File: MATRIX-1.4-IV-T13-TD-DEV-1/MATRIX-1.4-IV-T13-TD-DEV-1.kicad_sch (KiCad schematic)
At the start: 163 parts, among them Q401 MPSA42, Q402 MPSA42, Q403 MPSA92, Q404 MPSA92, Q405 MJE340, Q406 MJE350, Q407 MJE350, Q408 MJE340, Q409 MJE15032, Q410 MJE15033, Q411 2SC5200, Q412 2SA1943, Q4131 2SC5200, Q41310 2SC5200, Q4132 2SC5200, Q4133 2SC5200, Q4134 2SC5200, Q4135 2SC5200, Q4136 2SC5200, Q4137 2SC5200, Q4138 2SC5200, Q4139 2SC5200, Q4141 2SA1943, Q41410 2SA1943, Q4142 2SA1943, Q4143 2SA1943, Q4144 2SA1943, Q4145 2SA1943, Q4146 2SA1943, Q4147 2SA1943, Q4148 2SA1943, Q4149 2SA1943, Q601 2N5401, Q602 MJE340, Q603 MJE15032, Q604 2SC5200, Q605 2N5401, Q606 MJE340, Q607 2N5401, Q608 2N5401, Q701 2N5551, Q702 MJE350, Q703 MJE15033, Q704 2SA1943, Q705 2N5551, Q706 MJE350, Q707 2N5551, Q708 2N5551

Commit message: Routine Update Fri Jul 15 09:37:09 AM WIB 2022
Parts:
- L601, L701: footprint (none) -> MATRIX_1.4:TOROIDAL_INDUCTOR_0077083A7
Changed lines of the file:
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@@
     (stroke (width 0) (type default) (color 0 0 0 0))
   )
-  (wire (pts (xy 234.95 55.88) (xy 234.95 63.5))
-    (stroke (width 0) (type default) (color 0 0 0 0))
-  )
   (wire (pts (xy 63.5 181.61) (xy 63.5 184.15))
     (stroke (width 0) (type default) (color 0 0 0 0))
@@
     (stroke (width 0) (type default) (color 0 0 0 0))
   )
+  (wire (pts (xy 234.95 55.88) (xy 234.95 63.5))
+    (stroke (width 0) (type default) (color 0 0 0 0))
+  )
   (wire (pts (xy 317.5 111.76) (xy 317.5 115.57))
     (stroke (width 0) (type default) (color 0 0 0 0))
@@
     (property "Reference" "L701" (id 0) (at 336.55 157.48 90))
     (property "Value" "10uH" (id 1) (at 336.55 160.02 90))
-    (property "Footprint" "" (id 2) (at 336.55 152.4 0)
+    (property "Footprint" "MATRIX_1.4:TOROIDAL_INDUCTOR_0077083A7" (id 2) (at 336.55 152.4 0)
       (effects (font (size 1.27 1.27)) hide)
     )
@@
     (property "Reference" "L601" (id 0) (at 336.55 43.18 90))
     (property "Value" "10uH" (id 1) (at 336.55 45.72 90))
-    (property "Footprint" "" (id 2) (at 336.55 50.8 0)
+    (property "Footprint" "MATRIX_1.4:TOROIDAL_INDUCTOR_0077083A7" (id 2) (at 336.55 50.8 0)
       (effects (font (size 1.27 1.27)) hide)
     )

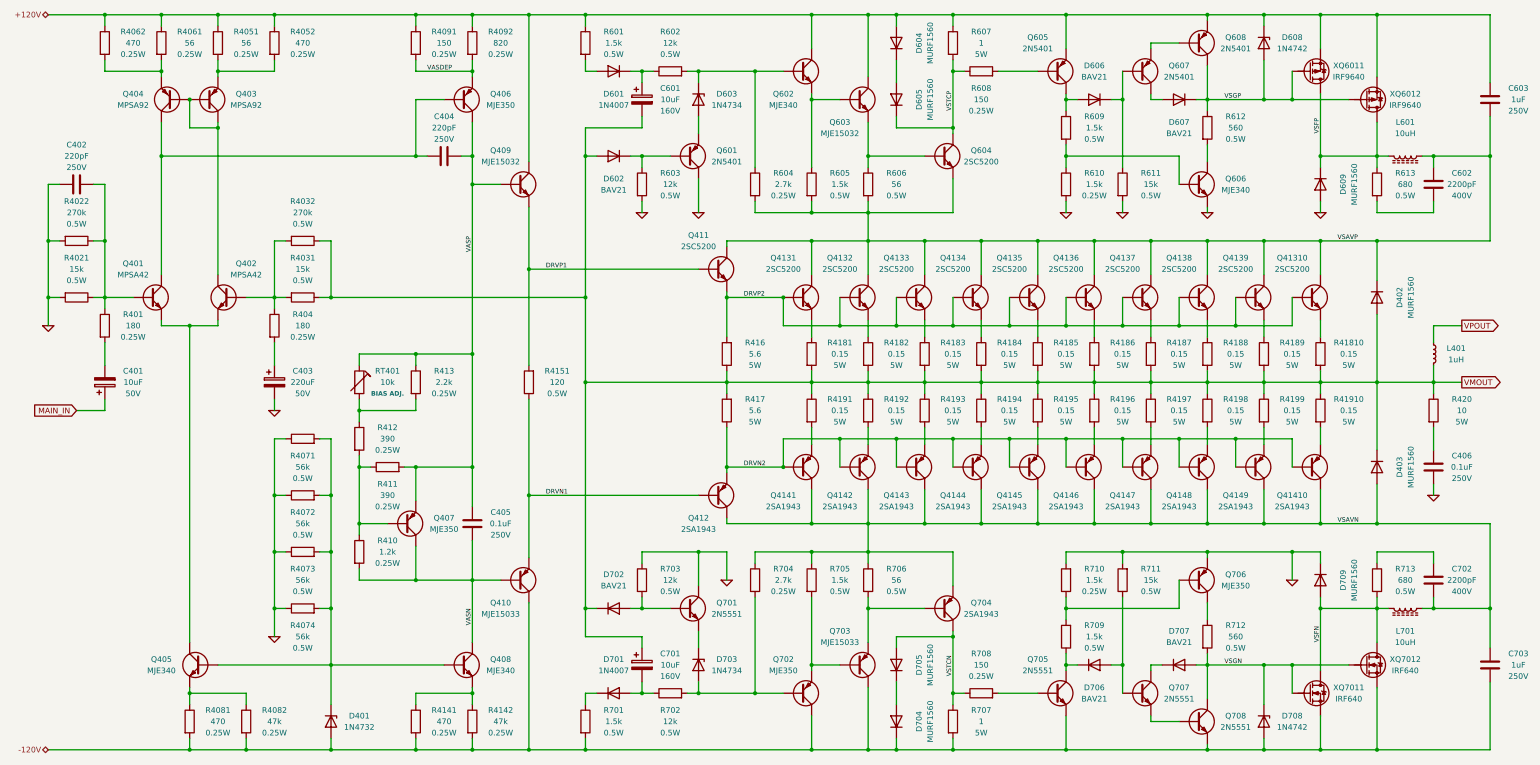
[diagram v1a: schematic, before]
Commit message: Routine Update Sat Jul 16 10:11:34 AM WIB 2022
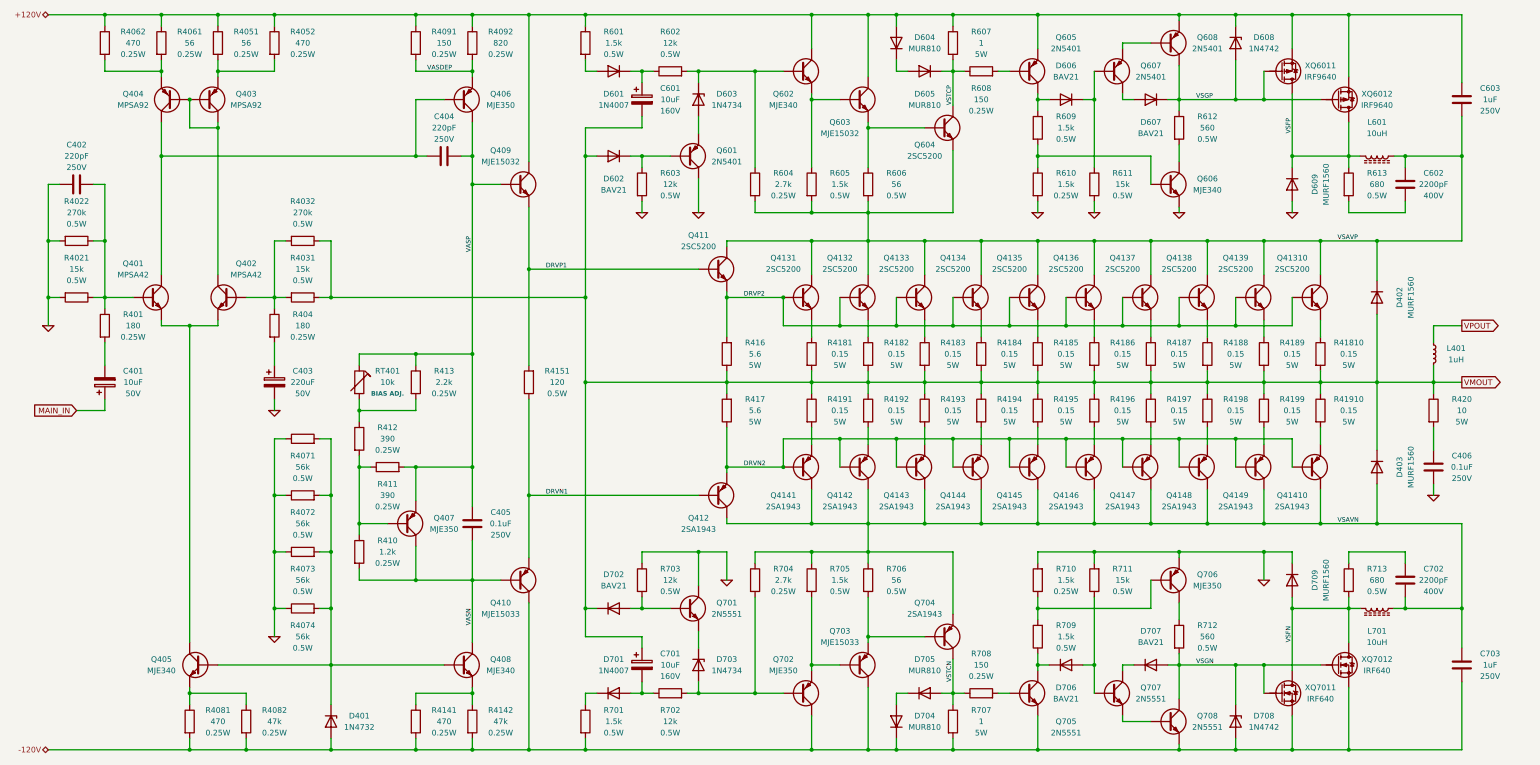
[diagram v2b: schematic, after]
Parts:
- D604, D605, D704, D705: value MURF1560 -> MUR810; Spice_Model MURF1560 -> MUR810
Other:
- moved on the sheet: C602, C603, C702, C703, D605, D606, D607, D608, D609, D705, D706, D707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
